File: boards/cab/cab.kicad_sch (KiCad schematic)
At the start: 39 parts, among them J1 Conn_01x08_Female, J2 Conn_01x08_Female, J3 Conn_01x08_Female, J4 Conn_01x08_Female, Q1 SI2308A, Q2 S8550, Q3 BC817-40,215, Q4 S8550, Q5 BC817-40,215, Q6 S8550, Q7 BC817-40,215, Q8 S8550, U1 XL1509-ADJ, U2 XL1509-5.0, U3 ATTINY1616-MNR

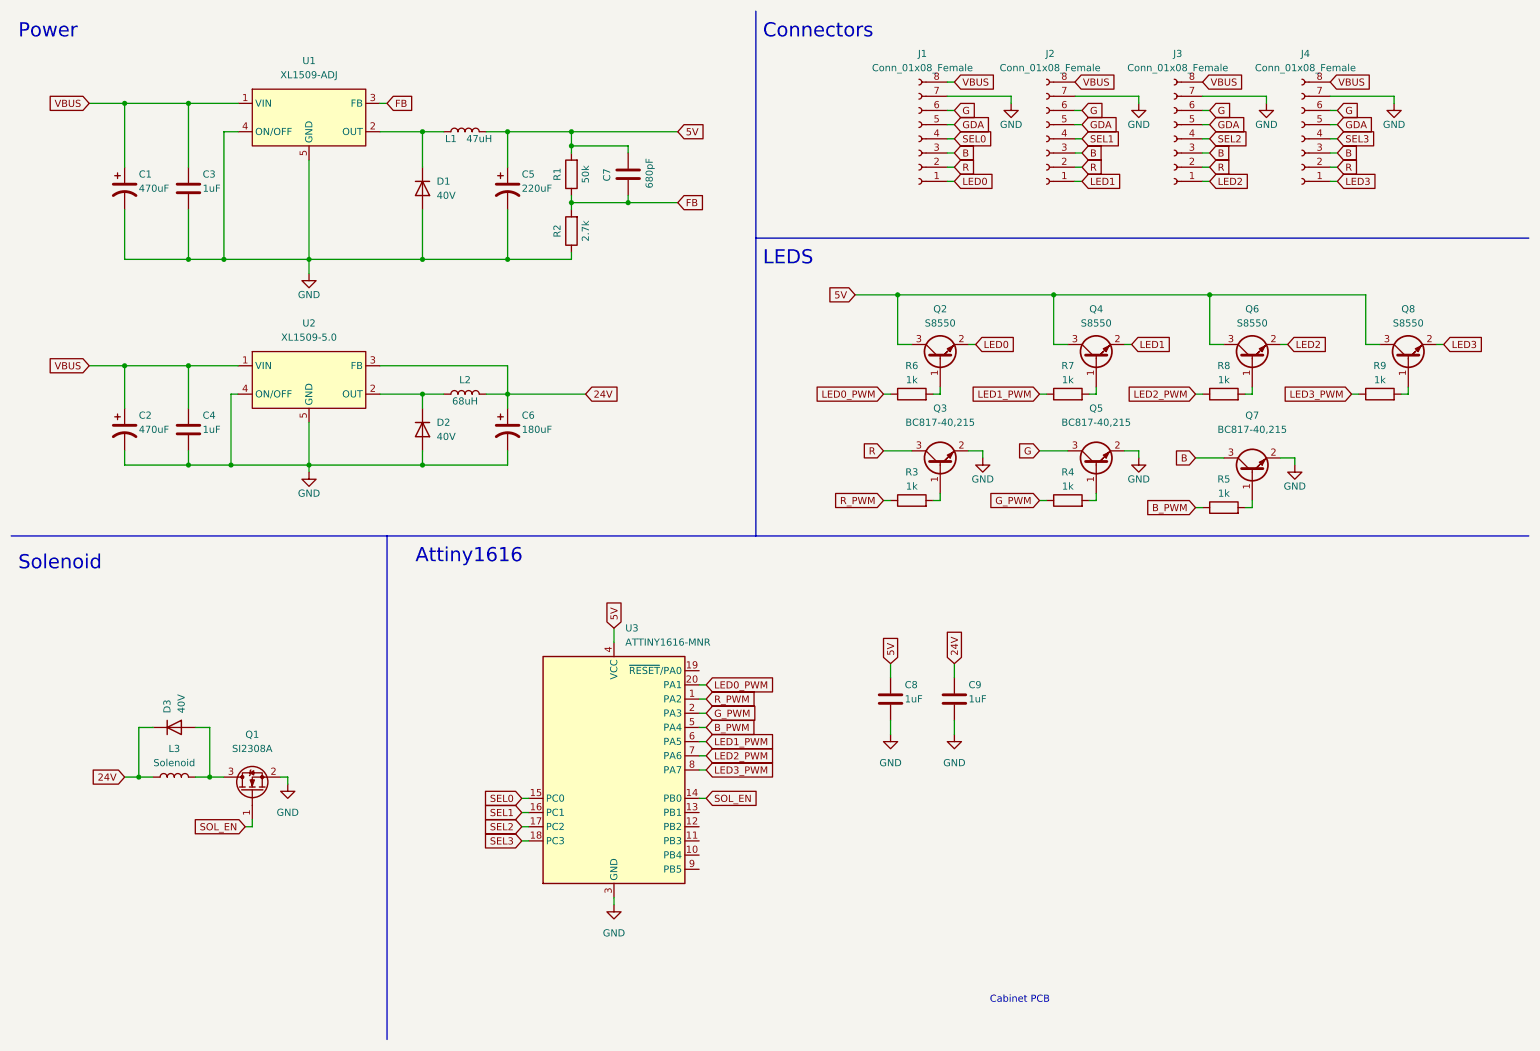
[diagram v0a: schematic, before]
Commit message: Created PCB
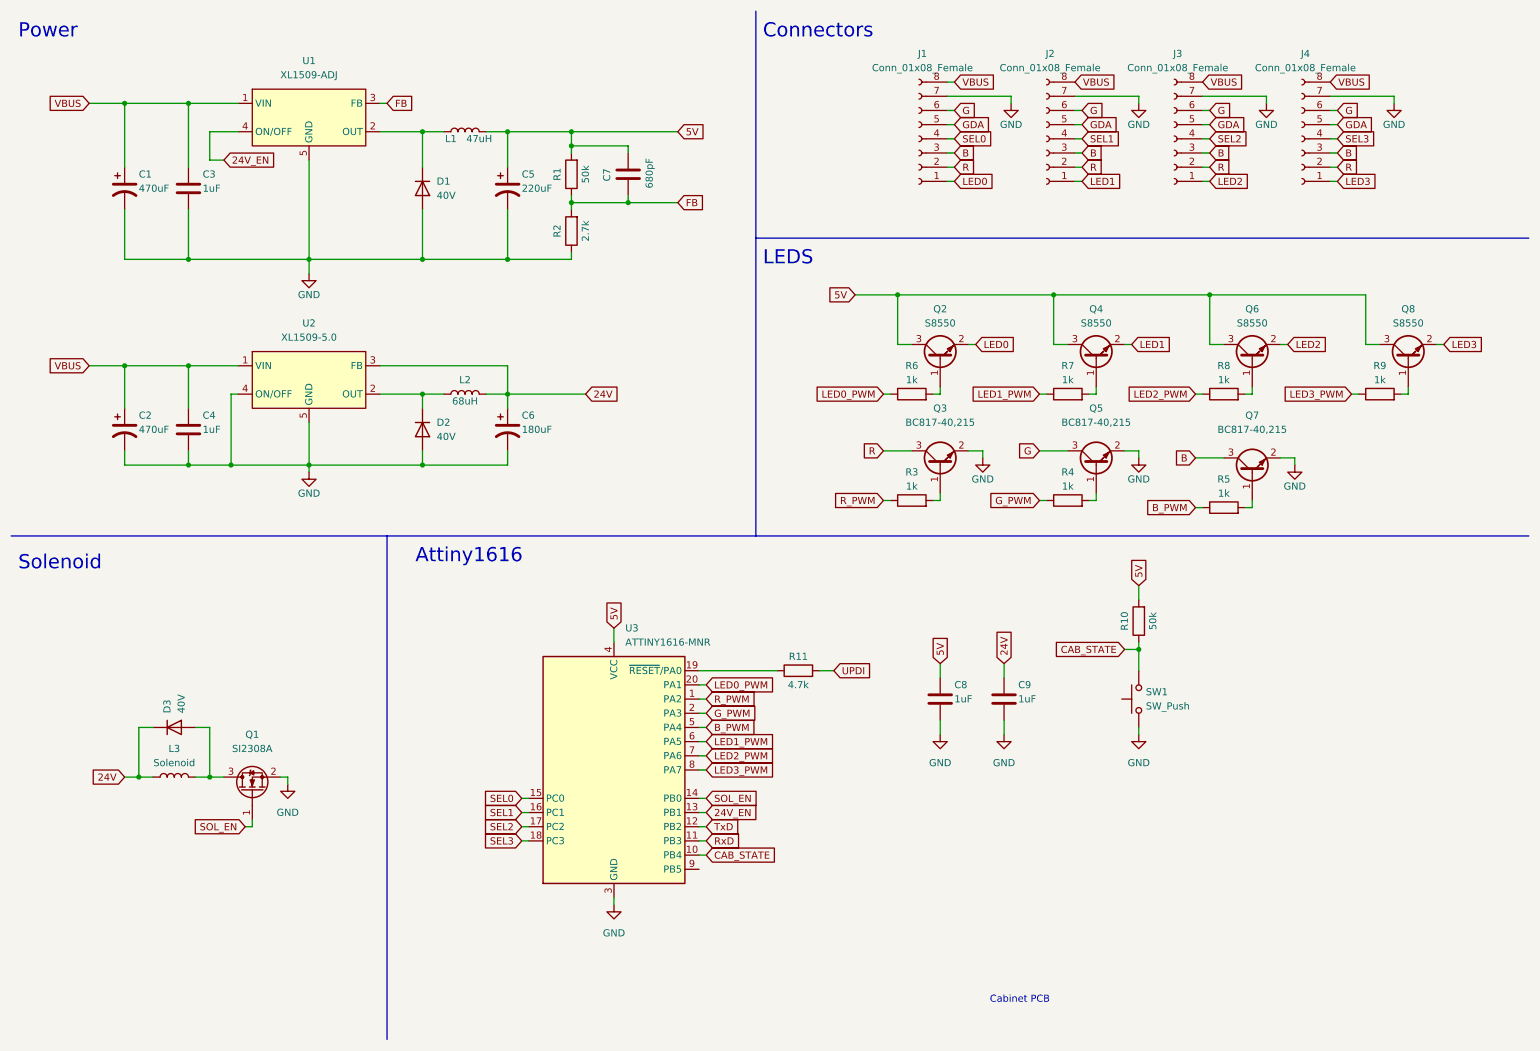
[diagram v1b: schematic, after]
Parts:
- added R10: 50k, Resistor_SMD:R_0805_2012Metric, symbol Device:R
- added R11: 4.7k, Resistor_SMD:R_0805_2012Metric, symbol Device:R
- added SW1: SW_Push, Connector_PinHeader_2.54mm:PinHeader_1x02_P2.54mm_Vertical, symbol Switch:SW_Push
- L3: footprint StackCabinet:Solenoid -> TerminalBlock_4Ucon:TerminalBlock_4Ucon_1x02_P3.50mm_Vertical; LCSC. Part# (none) -> C474892; Mfr. Part# (none) -> KF350-3.5-2P
- Q2, Q3, Q4, Q5, Q6, Q7, Q8: footprint Package_TO_SOT_THT:TO-220-3_Vertical -> Package_TO_SOT_SMD:SOT-23
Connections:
- net 5V: now also R10.2
- net GND: now also SW1.1; no longer U1.4 (ON/OFF)
- net CAB_STATE: now reaches U3.10 (PB4)
- net CAB_STATE: now also R10.1, SW1.2
- net RxD: now reaches U3.11 (PB3)
- net TxD: now reaches U3.12 (PB2)
- net 24V_EN: now reaches U3.13 (PB1)
- net 24V_EN: now also U1.4 (ON/OFF)
- net at U3.19 (~{RESET}/PA0): now also R11.1
- new net UPDI: R11.2
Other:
- moved on the sheet: C8, C9
